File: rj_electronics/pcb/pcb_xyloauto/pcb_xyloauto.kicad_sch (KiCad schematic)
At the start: 7 parts

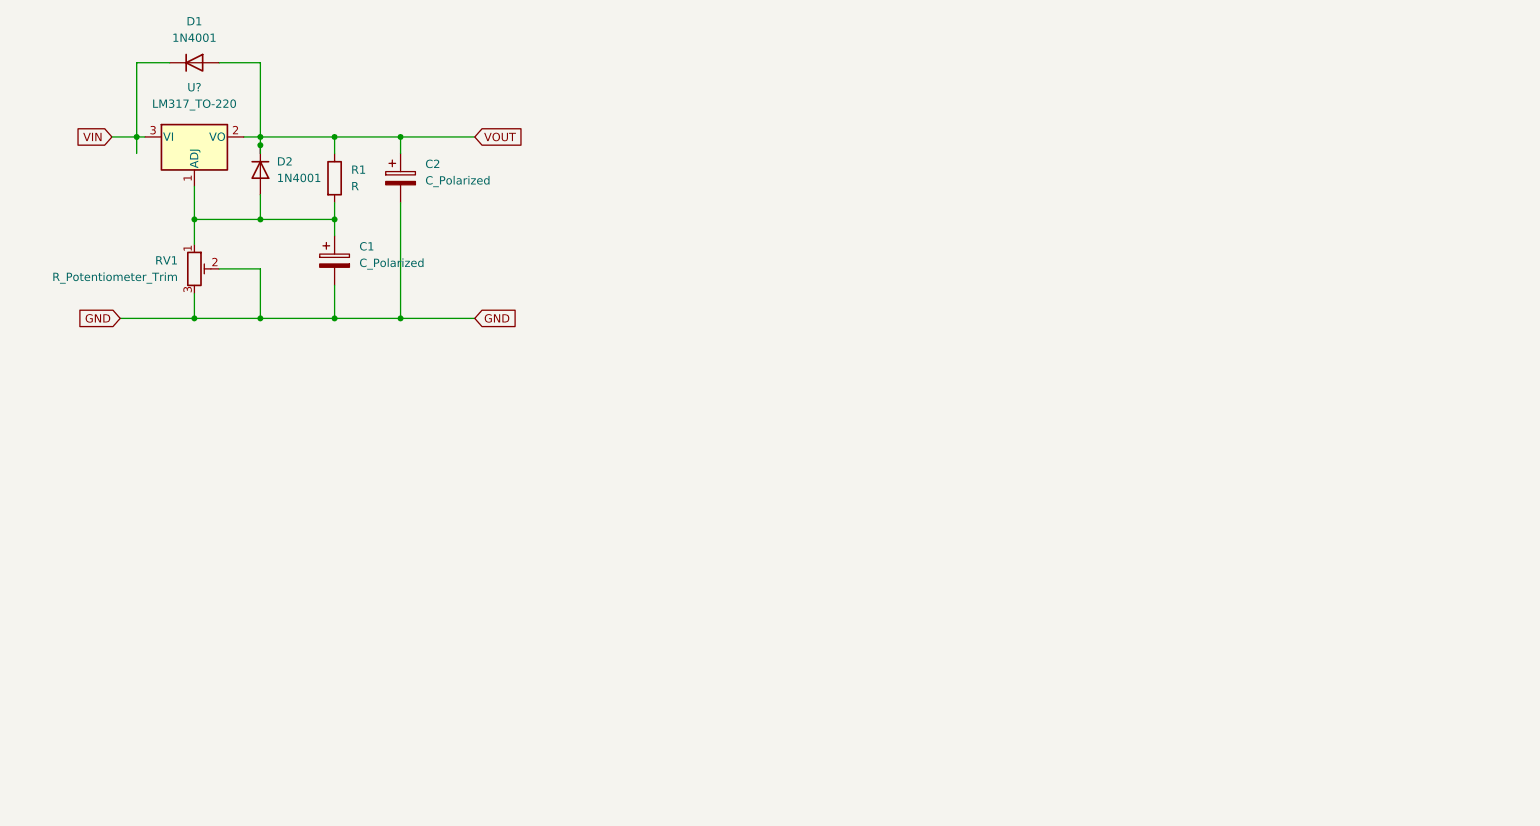
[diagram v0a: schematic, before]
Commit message: nc
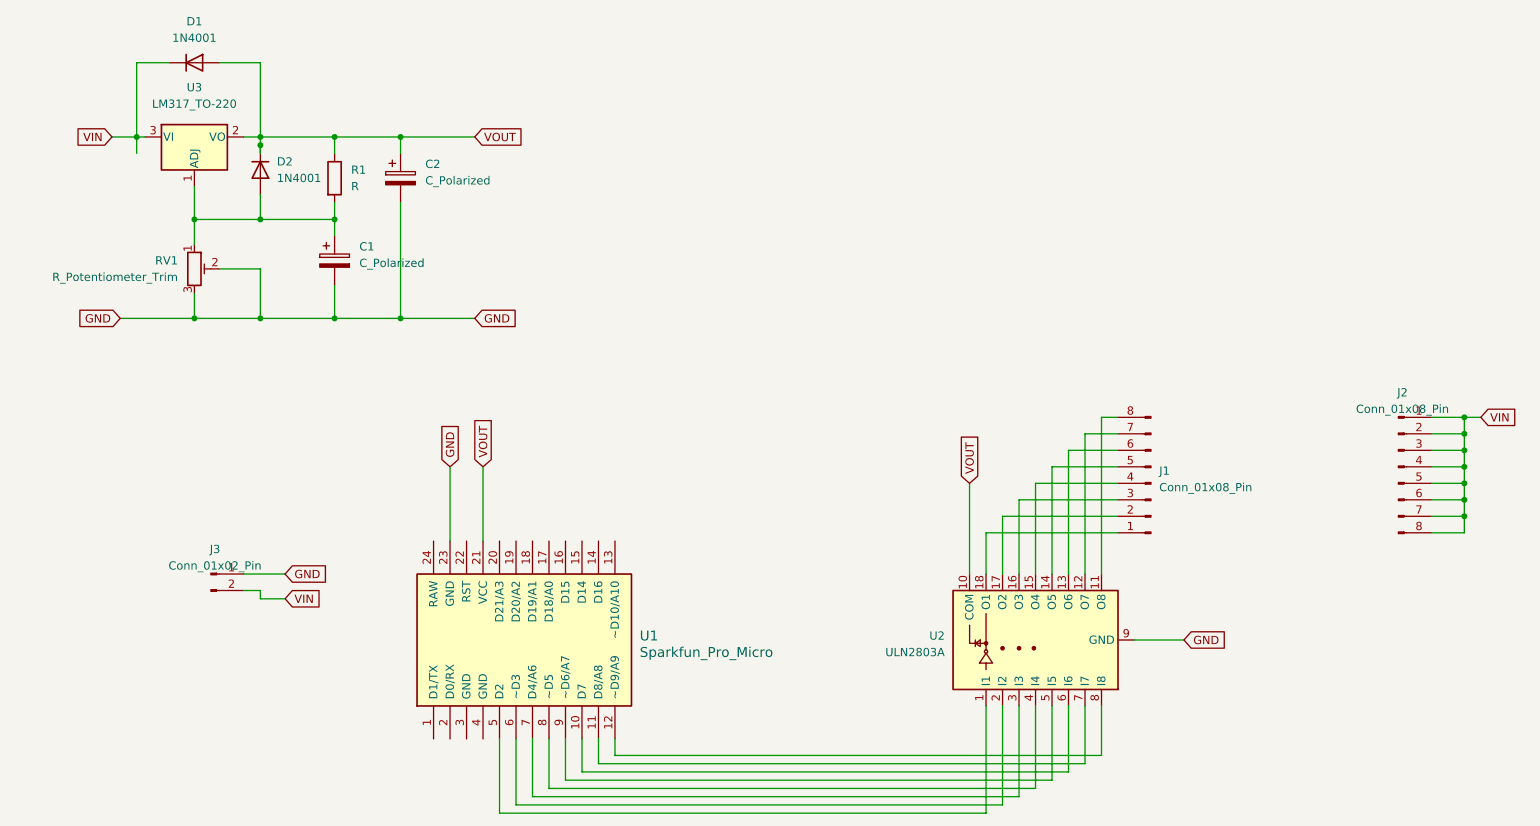
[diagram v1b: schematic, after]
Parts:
- added J1, J2: Conn_01x08_Pin, Connector_PinSocket_2.54mm:PinSocket_1x08_P2.54mm_Vertical, symbol Connector:Conn_01x08_Pin
- added J3: Conn_01x02_Pin, Connector_PinHeader_2.54mm:PinHeader_1x02_P2.54mm_Vertical, symbol Connector:Conn_01x02_Pin
- added U1: Sparkfun_Pro_Micro, Arduino:Sparkfun_Pro_Micro, symbol Arduino:Sparkfun_Pro_Micro
- added U2: ULN2803A, Package_DIP:DIP-18_W7.62mm_Socket, symbol Transistor_Array:ULN2803A
- C2: footprint (none) -> Capacitor_THT:CP_Radial_D10.0mm_P2.50mm
- gave numbers to parts that had none: 1
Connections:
- net GND: now also J3.1 (Pin_1), U1.23 (GND), U2.9 (GND)
- net VIN: now also J2.1 (Pin_1), J2.2 (Pin_2), J2.3 (Pin_3), J2.4 (Pin_4), J2.5 (Pin_5), J2.6 (Pin_6), J2.7 (Pin_7), J2.8 (Pin_8), J3.2 (Pin_2)
- net VOUT: now also U1.21 (VCC), U2.10 (COM)
- new net: U1.5 (D2), U2.1 (I1)
- new net: J1.8 (Pin_8), U2.11 (O8)
- new net: J1.7 (Pin_7), U2.12 (O7)
- new net: J1.6 (Pin_6), U2.13 (O6)
- new net: J1.5 (Pin_5), U2.14 (O5)
- new net: J1.4 (Pin_4), U2.15 (O4)
- new net: J1.3 (Pin_3), U2.16 (O3)
- new net: J1.2 (Pin_2), U2.17 (O2)
- new net: J1.1 (Pin_1), U2.18 (O1)
- new net: U1.6 (~D3), U2.2 (I2)
- new net: U1.7 (D4/A6), U2.3 (I3)
- new net: U1.8 (~D5), U2.4 (I4)
- new net: U1.9 (~D6/A7), U2.5 (I5)
- new net: U1.10 (D7), U2.6 (I6)
- new net: U1.11 (D8/A8), U2.7 (I7)
- new net: U1.12 (~D9/A9), U2.8 (I8)
